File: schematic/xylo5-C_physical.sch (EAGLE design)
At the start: 53 parts, among them IC1 ATMEGA88, IC2 Si4362, P10 MA01-1, P9 MA01-1, X1 8M10AHC49T

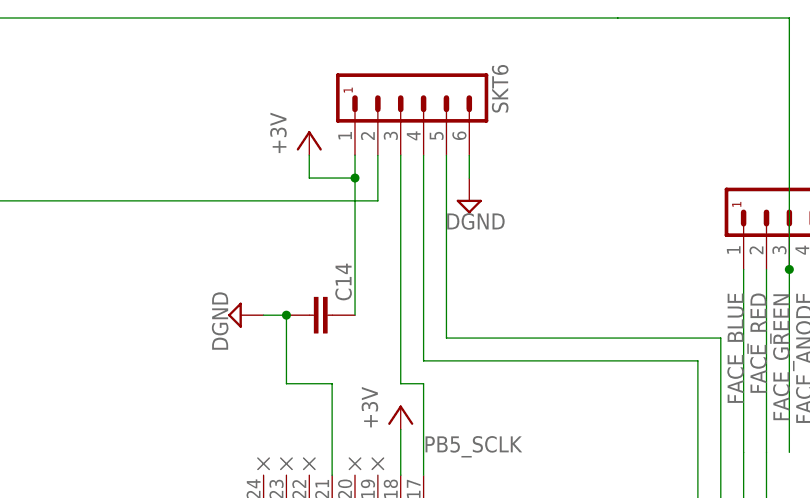
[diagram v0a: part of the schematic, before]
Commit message: Add some net labels.
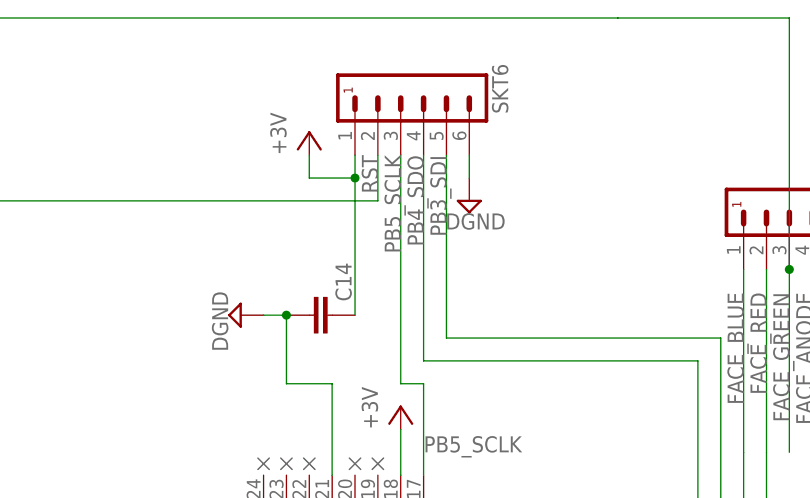
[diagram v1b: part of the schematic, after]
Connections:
- net N$1 renamed RST
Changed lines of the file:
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@@
 </segment>
 </net>
-<net name="N$1" class="0">
+<net name="RST" class="0">
 <segment>
 <pinref part="C16" gate="G$1" pin="1"/>
@@
 <wire x1="134.62" y1="170.18" x2="116.84" y2="170.18" width="0.1524" layer="91"/>
 <junction x="116.84" y="170.18"/>
+<label x="162.56" y="231.14" size="1.778" layer="95" rot="MR270"/>
 </segment>
 </net>
@@
 <pinref part="SKT6" gate="G$1" pin="5"/>
 <wire x1="170.18" y1="210.82" x2="170.18" y2="231.14" width="0.1524" layer="91"/>
+<label x="170.18" y="231.14" size="1.778" layer="95" rot="MR270"/>
 </segment>
 </net>
@@
 <wire x1="167.64" y1="208.28" x2="198.12" y2="208.28" width="0.1524" layer="91"/>
 <wire x1="198.12" y1="208.28" x2="198.12" y2="180.34" width="0.1524" layer="91"/>
+<label x="167.64" y="231.14" size="1.778" layer="95" rot="MR270"/>
 </segment>
 <segment>
@@
 <wire x1="167.64" y1="205.74" x2="167.64" y2="195.58" width="0.1524" layer="91"/>
 <label x="167.64" y="198.12" size="1.778" layer="95"/>
-</segment>
-<segment>
+<label x="165.1" y="231.14" size="1.778" layer="95" rot="MR270"/>
+</segment>
+<segment>

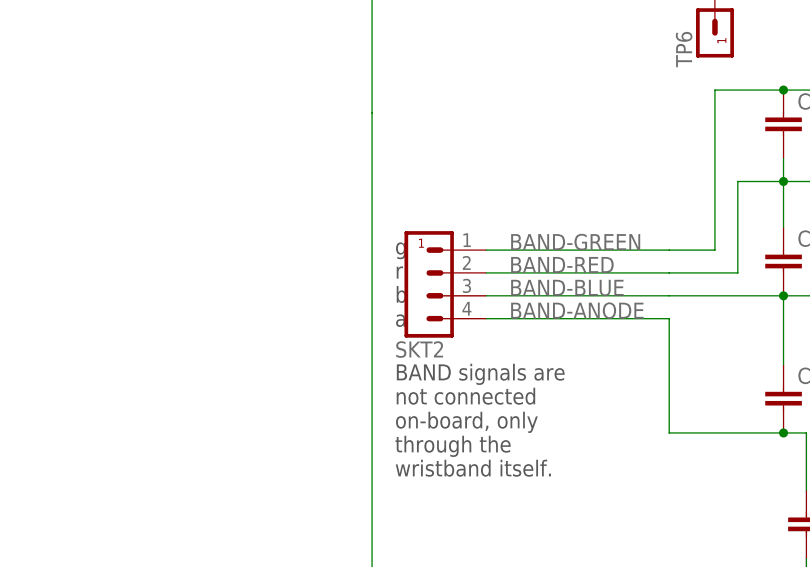
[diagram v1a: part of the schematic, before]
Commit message: Remove leftover note.
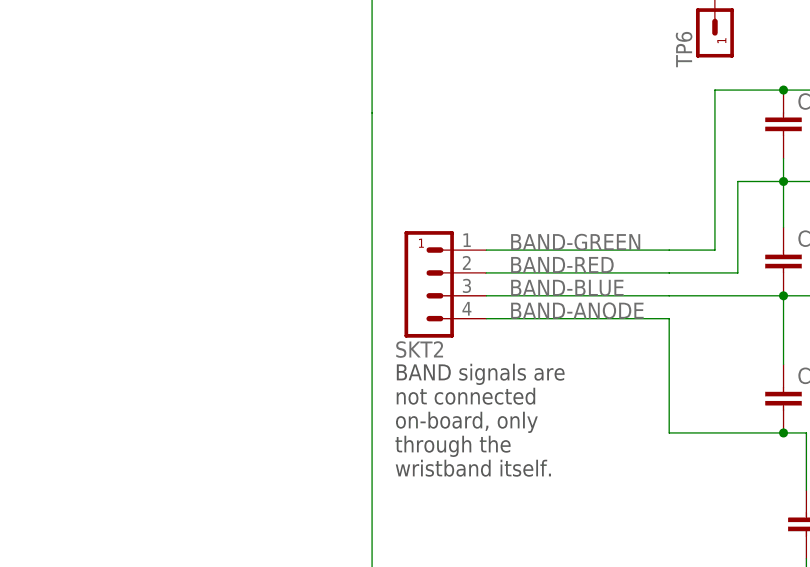
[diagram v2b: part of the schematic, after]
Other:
- note removed: "g r b a"
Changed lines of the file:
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@@
 <wire x1="132.715" y1="172.085" x2="133.985" y2="173.355" width="0.1524" layer="97"/>
 <wire x1="133.985" y1="172.085" x2="132.715" y2="173.355" width="0.1524" layer="97"/>
-<text x="63.5" y="67.31" size="1.778" layer="97" align="top-left">g
-r
-b
-a</text>
 <text x="166.37" y="31.75" size="1.27" layer="97" align="top-left">This is just my
 BEST GUESS of

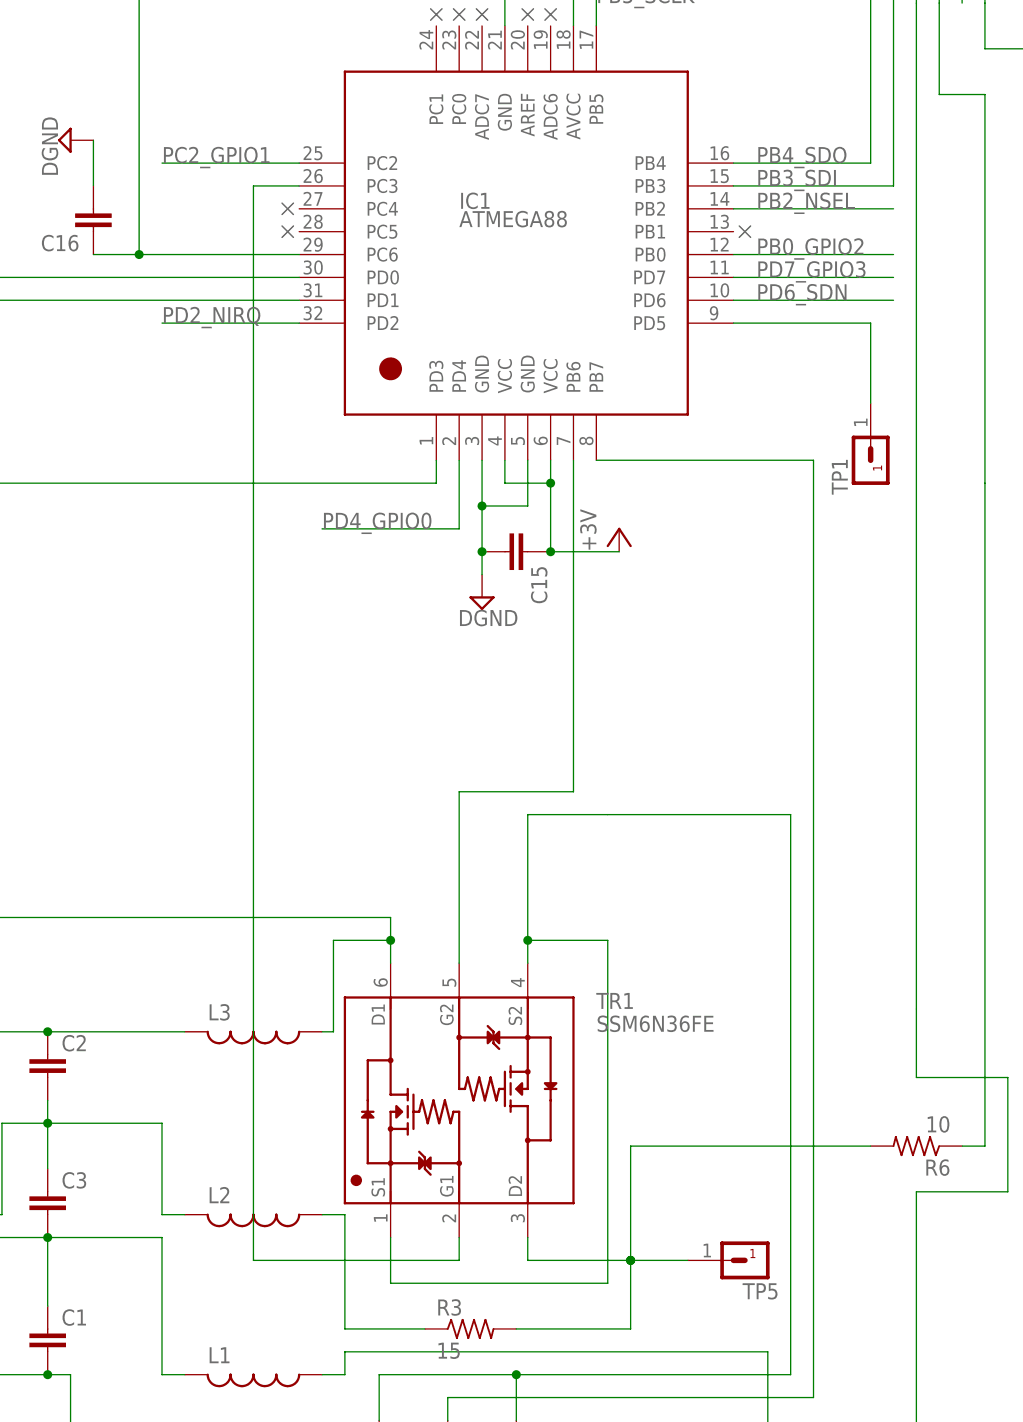
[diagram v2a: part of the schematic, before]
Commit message: Add some net labels.
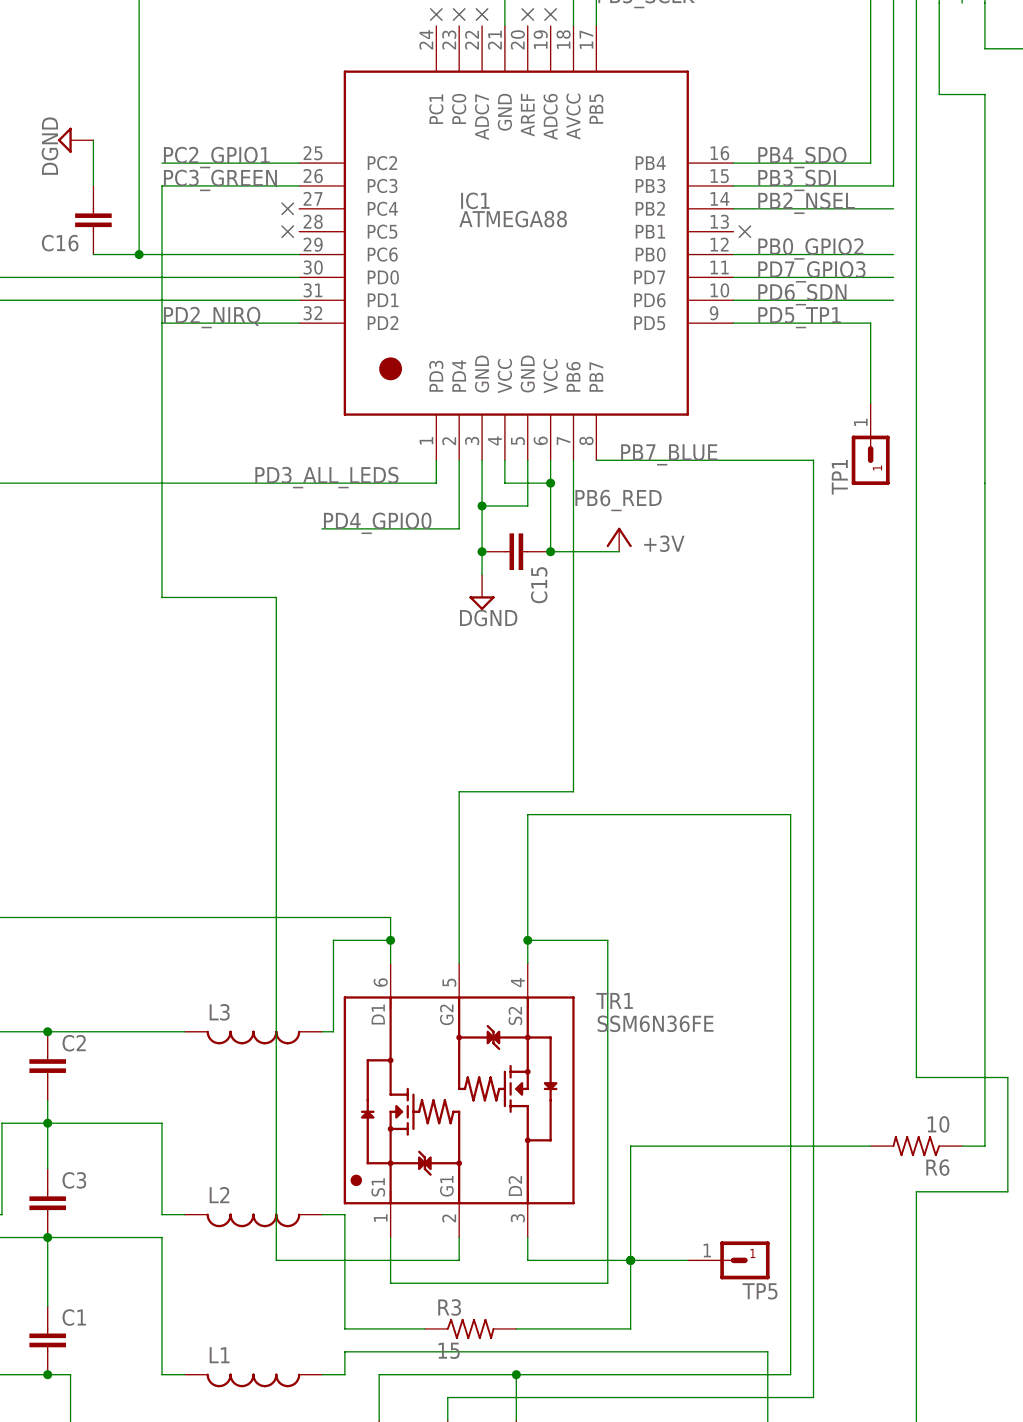
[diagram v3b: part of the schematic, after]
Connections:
- net N$11 renamed PD3_ALL_LEDS
- net N$18 renamed PB7_BLUE
- net N$20 renamed PB6_RED
- net N$22 renamed PC3_GREEN
- net N$9 renamed PD5_TP1
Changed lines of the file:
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@@
 <instance part="P+6" gate="VCC" x="154.94" y="233.68"/>
 <instance part="P+1" gate="VCC" x="165.1" y="203.2"/>
-<instance part="P+2" gate="VCC" x="170.18" y="139.7"/>
+<instance part="P+2" gate="VCC" x="170.18" y="139.7" smashed="yes">
+<attribute name="VALUE" x="172.72" y="137.16" size="1.778" layer="96"/>
+</instance>
 <instance part="P+7" gate="G$1" x="195.58" y="-12.7"/>
 <instance part="P+8" gate="G$1" x="220.98" y="66.04"/>
@@
 </segment>
 </net>
-<net name="N$11" class="0">
+<net name="PD3_ALL_LEDS" class="0">
 <segment>
 <pinref part="TP7" gate="G$1" pin="1"/>
@@
 <wire x1="149.86" y1="144.78" x2="149.86" y2="147.32" width="0.1524" layer="91"/>
 <pinref part="TR2" gate="G$1" pin="G2"/>
+<label x="129.54" y="144.78" size="1.778" layer="95"/>
 </segment>
 </net>
@@
 </segment>
 </net>
-<net name="N$18" class="0">
+<net name="PB7_BLUE" class="0">
 <segment>
 <wire x1="151.13" y1="40.64" x2="151.13" y2="43.18" width="0.1524" layer="91"/>
@@
 <wire x1="191.77" y1="147.32" x2="167.64" y2="147.32" width="0.1524" layer="91"/>
 <pinref part="TR2" gate="G$1" pin="G1"/>
-</segment>
-</net>
-<net name="N$20" class="0">
+<label x="170.18" y="147.32" size="1.778" layer="95"/>
+</segment>
+</net>
+<net name="PB6_RED" class="0">
 <segment>
 <wire x1="165.1" y1="110.49" x2="152.4" y2="110.49" width="0.1524" layer="91"/>
@@
 <wire x1="165.1" y1="110.49" x2="165.1" y2="147.32" width="0.1524" layer="91"/>
 <pinref part="TR1" gate="G$1" pin="G2"/>
-</segment>
-</net>
-<net name="N$22" class="0">
+<label x="165.1" y="142.24" size="1.778" layer="95"/>
+</segment>
+</net>
+<net name="PC3_GREEN" class="0">
 <segment>
 <pinref part="IC1" gate="G$1" pin="PC3"/>
-<wire x1="134.62" y1="177.8" x2="129.54" y2="177.8" width="0.1524" layer="91"/>
-<wire x1="129.54" y1="177.8" x2="129.54" y2="58.42" width="0.1524" layer="91"/>
-<wire x1="129.54" y1="58.42" x2="152.4" y2="58.42" width="0.1524" layer="91"/>
+<wire x1="134.62" y1="177.8" x2="132.08" y2="177.8" width="0.1524" layer="91"/>
+<wire x1="132.08" y1="177.8" x2="119.38" y2="177.8" width="0.1524" layer="91"/>
+<wire x1="119.38" y1="177.8" x2="119.38" y2="132.08" width="0.1524" layer="91"/>
+<wire x1="119.38" y1="132.08" x2="132.08" y2="132.08" width="0.1524" layer="91"/>
+<wire x1="132.08" y1="132.08" x2="132.08" y2="58.42" width="0.1524" layer="91"/>
+<wire x1="132.08" y1="58.42" x2="152.4" y2="58.42" width="0.1524" layer="91"/>
 <pinref part="TR1" gate="G$1" pin="G1"/>
 <wire x1="152.4" y1="58.42" x2="152.4" y2="60.96" width="0.1524" layer="91"/>
+<label x="119.38" y="177.8" size="1.778" layer="95"/>
 </segment>
 </net>
@@
 </segment>
 </net>
-<net name="N$9" class="0">
+<net name="PD5_TP1" class="0">
 <segment>
 <pinref part="TP1" gate="G$1" pin="1"/>
@@
 <wire x1="198.12" y1="153.67" x2="198.12" y2="162.56" width="0.1524" layer="91"/>
 <wire x1="198.12" y1="162.56" x2="182.88" y2="162.56" width="0.1524" layer="91"/>
-</segment>
-</net>
+<label x="185.42" y="162.56" size="1.778" layer="95"/>
+</segment>
+</net>
